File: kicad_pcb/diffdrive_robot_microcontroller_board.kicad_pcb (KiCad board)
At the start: 2 copper layers, 86.4 x 53.8 mm, 24 parts, among them J0 Battery_Input, J1 Odom L, J10 digital_expansion, J11 external_hbridge, J12 Motor_Pins, J2 Odom R, J3 Sensor A, J4 Sensor B, J5 Sensor C, J6 Sensor D, J7 nRF24L01 Connector, J8 i2c accel/gyro, J9 analog_expansion, U1 Pico, U2 TB6612FNG, U3 Buck Converter, U4 LM393

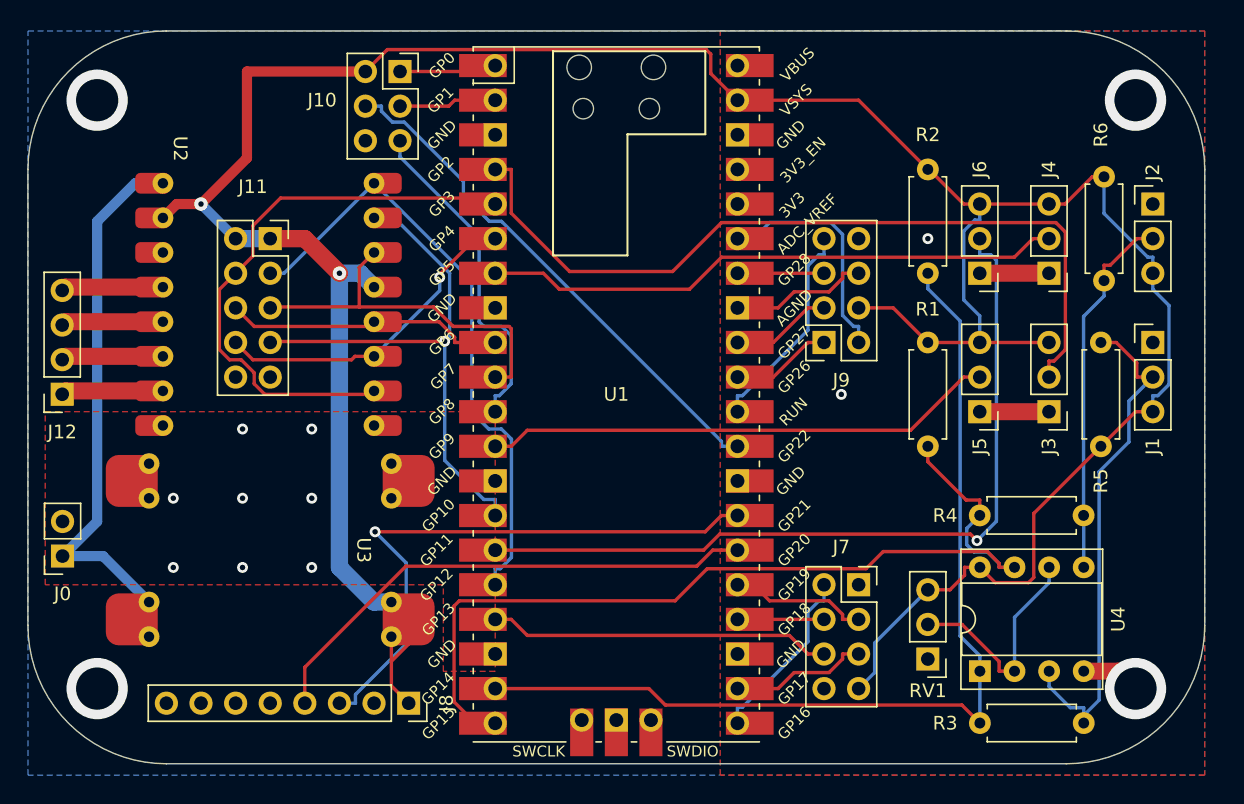
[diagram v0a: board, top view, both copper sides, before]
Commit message: August through October 2025 CAD revisions
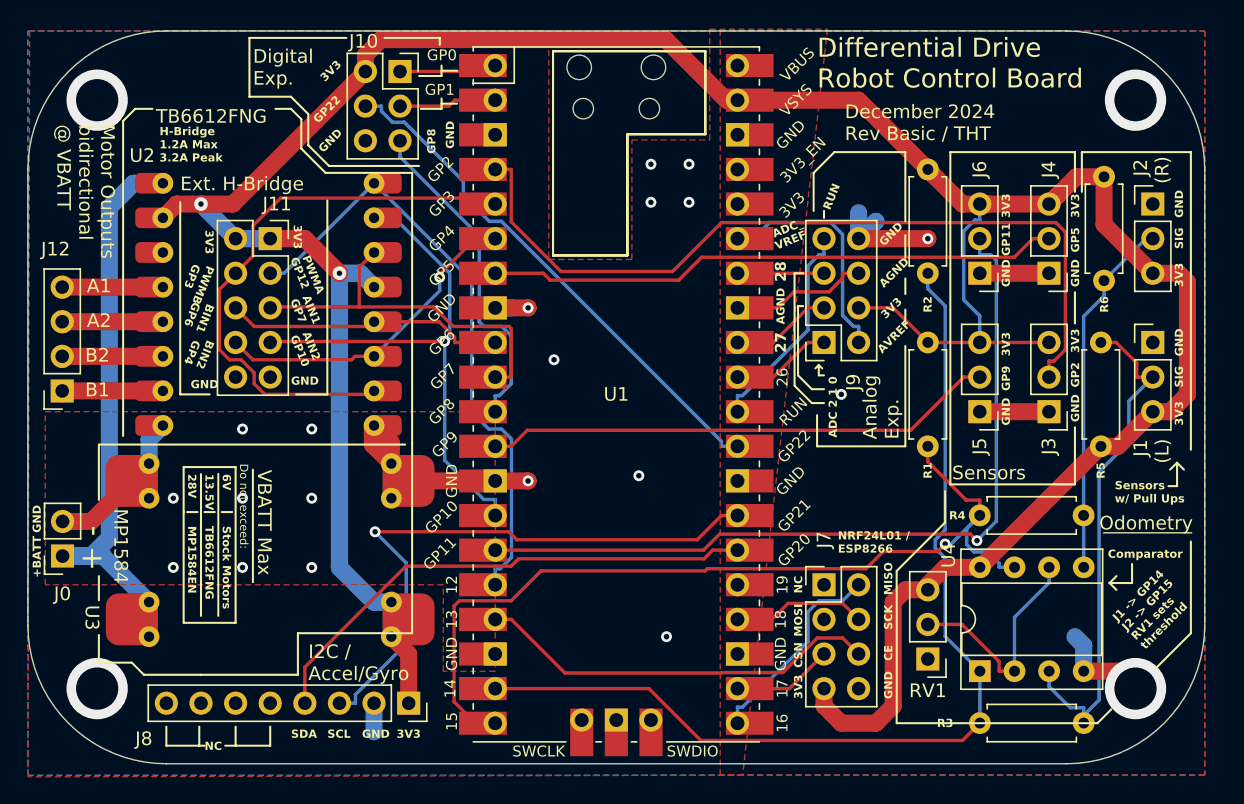
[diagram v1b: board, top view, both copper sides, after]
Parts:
- added G***: LOGO, simplebot:ffwf_logo_flames_1300dpi, B.Cu at (199.4, 79.4)
- added G***: LOGO, simplebot:ffwf_logo_1300dpi, B.Cu at (199.4, 79.4)
- added G1: LOGO, simplebot:BRS_LOGO, B.Cu at (173.8, 77.0)
- added G2: LOGO, simplebot:BRS_TEXT, B.Cu at (147.3, 75.8)
- added REF**: KiCad-Logo_5mm_SilkScreen, Symbol:KiCad-Logo_5mm_SilkScreen, B.Cu at (155.7, 90.0)
- added REF**: OSHW-Logo2_9.8x8mm_SilkScreen, Symbol:OSHW-Logo2_9.8x8mm_SilkScreen, B.Cu at (163.1, 92.3)
- J7: moved to B.Cu
- moved J7 2.54 mm to (175.3, 88.5), turned to 180 degrees
- moved J12 0.24 mm to (119.4, 74.2)
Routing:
- net GND: track 14.5 -> 65.7 mm, vias 14 -> 23
- net MOSI: track 10.2 -> 1.18 mm
- net +3V3: track 219.3 -> 224.7 mm
- net CE: track 25.2 -> 29.9 mm
- net SCK: track 6.35 -> 9.86 mm
- net CSN: track 10.2 -> 7.40 mm
- net Net-(U1-Pad20): track 68.3 -> 66.2 mm, vias 0 -> 1
- net MISO: track 13.2 -> 15.1 mm
- net Net-(U4-Pad1): track 71.2 -> 72.9 mm
- net +BATT: track 43.7 -> 45.0 mm
- net Net-(U4-Pad5): track 27.2 -> 26.5 mm
- net Net-(U1-Pad7): track 42.7 -> 42.1 mm
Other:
- board text added: "(L)"
- board text added: "(R)"
- board text added: "+"
- board text added: "+BATT"
- board text added: "-"
- board text added: "13.5V"
- board text added: "28V"
- board text added: "3V3"
- board text added: "6V"
- board text added: "A1"
- board text added: "A2"
- board text added: "ADC 2 1 0"
- board text added: "AGND"
- board text added: "AIN1"
- board text added: "AIN2"
- board text added: "AVREF"
- board text added: "Analog Exp."
- board text added: "B1"
- board text added: "B2"
- board text added: "BIN1"
- board text added: "BIN2"
- board text added: "CE"
- board text added: "CSN"
- board text added: "Comparator"
- board text added: "December 2024 Rev Basic / THT"
- board text added: "Differential Drive Robot Control Board"
- board text added: "Digital Exp."
- board text added: "Do not exceed:"
- board text added: "Ext. H-Bridge"
- board text added: "FFwF.net"
- board text added: "GND"
- board text added: "GP10"
- board text added: "GP11"
- board text added: "GP12"
- board text added: "GP2"
- board text added: "GP22"
- board text added: "GP3"
- board text added: "GP4"
- board text added: "GP5"
- board text added: "GP6"
- board text added: "GP7"
- board text added: "GP8"
- board text added: "GP9"
- board text added: "H-Bridge 1.2A Max 3.2A Peak"
- board text added: "I2C / Accel/Gyro"
- board text added: "J1 -> GP14 J2 -> GP15 RV1 sets threshold"
- board text added: "MISO"
- board text added: "MOSI"
- board text added: "MP1584"
- board text added: "MP1584EN"
- board text added: "Motor Outputs bidirectional @ VBATT"
- board text added: "NC"
- board text added: "NRF24L01 / ESP8266"
- board text added: "Odometry"
- board text added: "PWMA"
- board text added: "PWMB"
- board text added: "R5"
- board text added: "R6"
- board text added: "RUN"
- board text added: "SCHEMATIC, SILKSCREEN and THT LAYOUT by John McCardle SIR PENNYBOTTOM LOGO by Danny Ferbert Simplebot PCB project: Deliver 100 robots in 2025 or bust!"
- board text added: "SCK"
- board text added: "SCL"
- board text added: "SDA"
- board text added: "SIG"
- board text added: "Sensors"
- board text added: "Sensors w/ Pull Ups"
- board text added: "Sponsored by: Fight Fire with Fire Robotics"
- board text added: "Stock Motors"
- board text added: "TB6612FNG"
- board text added: "VBATT Max"
- board text added: "VREF"
- board text added: "{dblquote}Loyal automatons for the inevitable machine uprising{dblquote}"
